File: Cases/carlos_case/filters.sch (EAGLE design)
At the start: 93 parts, among them IC1 NE5532N, IC2 NE5532N, IC3 NE5532N, IC4 NE5532N, IC5 NE5532N, IC6 NE5532N, IC7 NE5532N, J1 3_PIN_AMPCONN, J2 4_PIN_AMPCONN

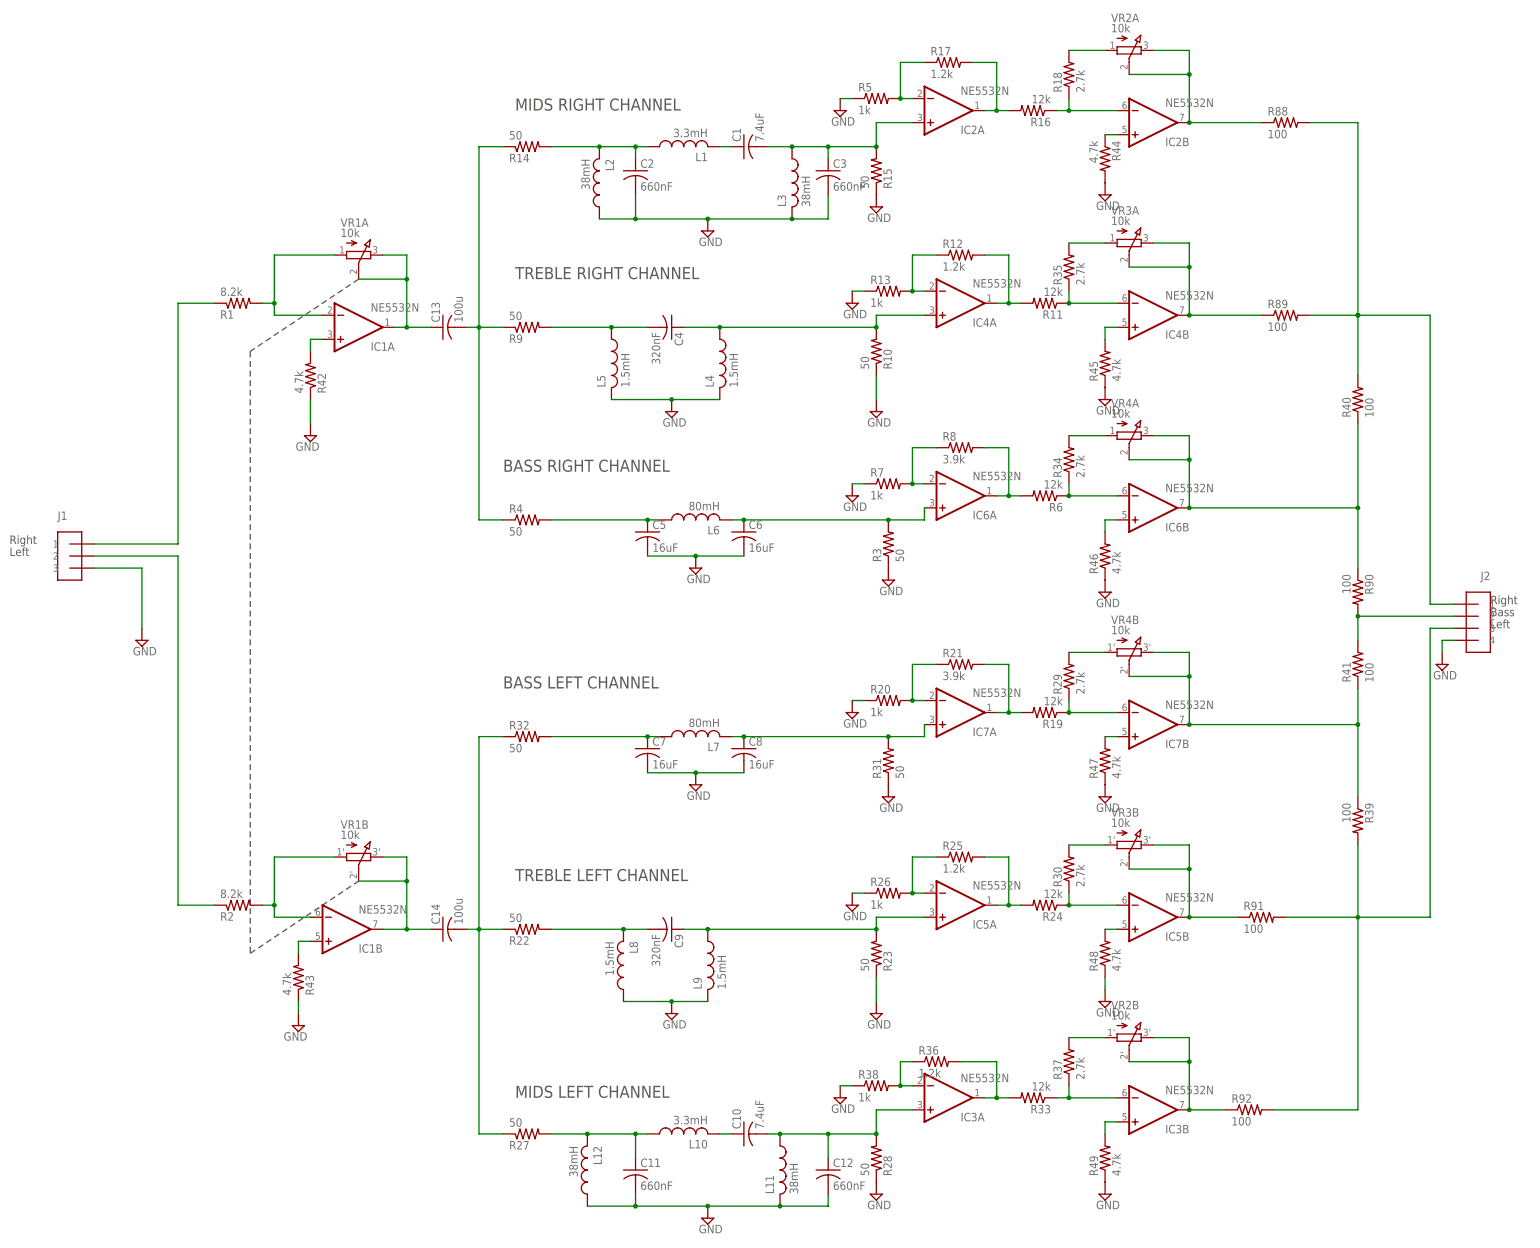
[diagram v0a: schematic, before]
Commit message: added folder for my case
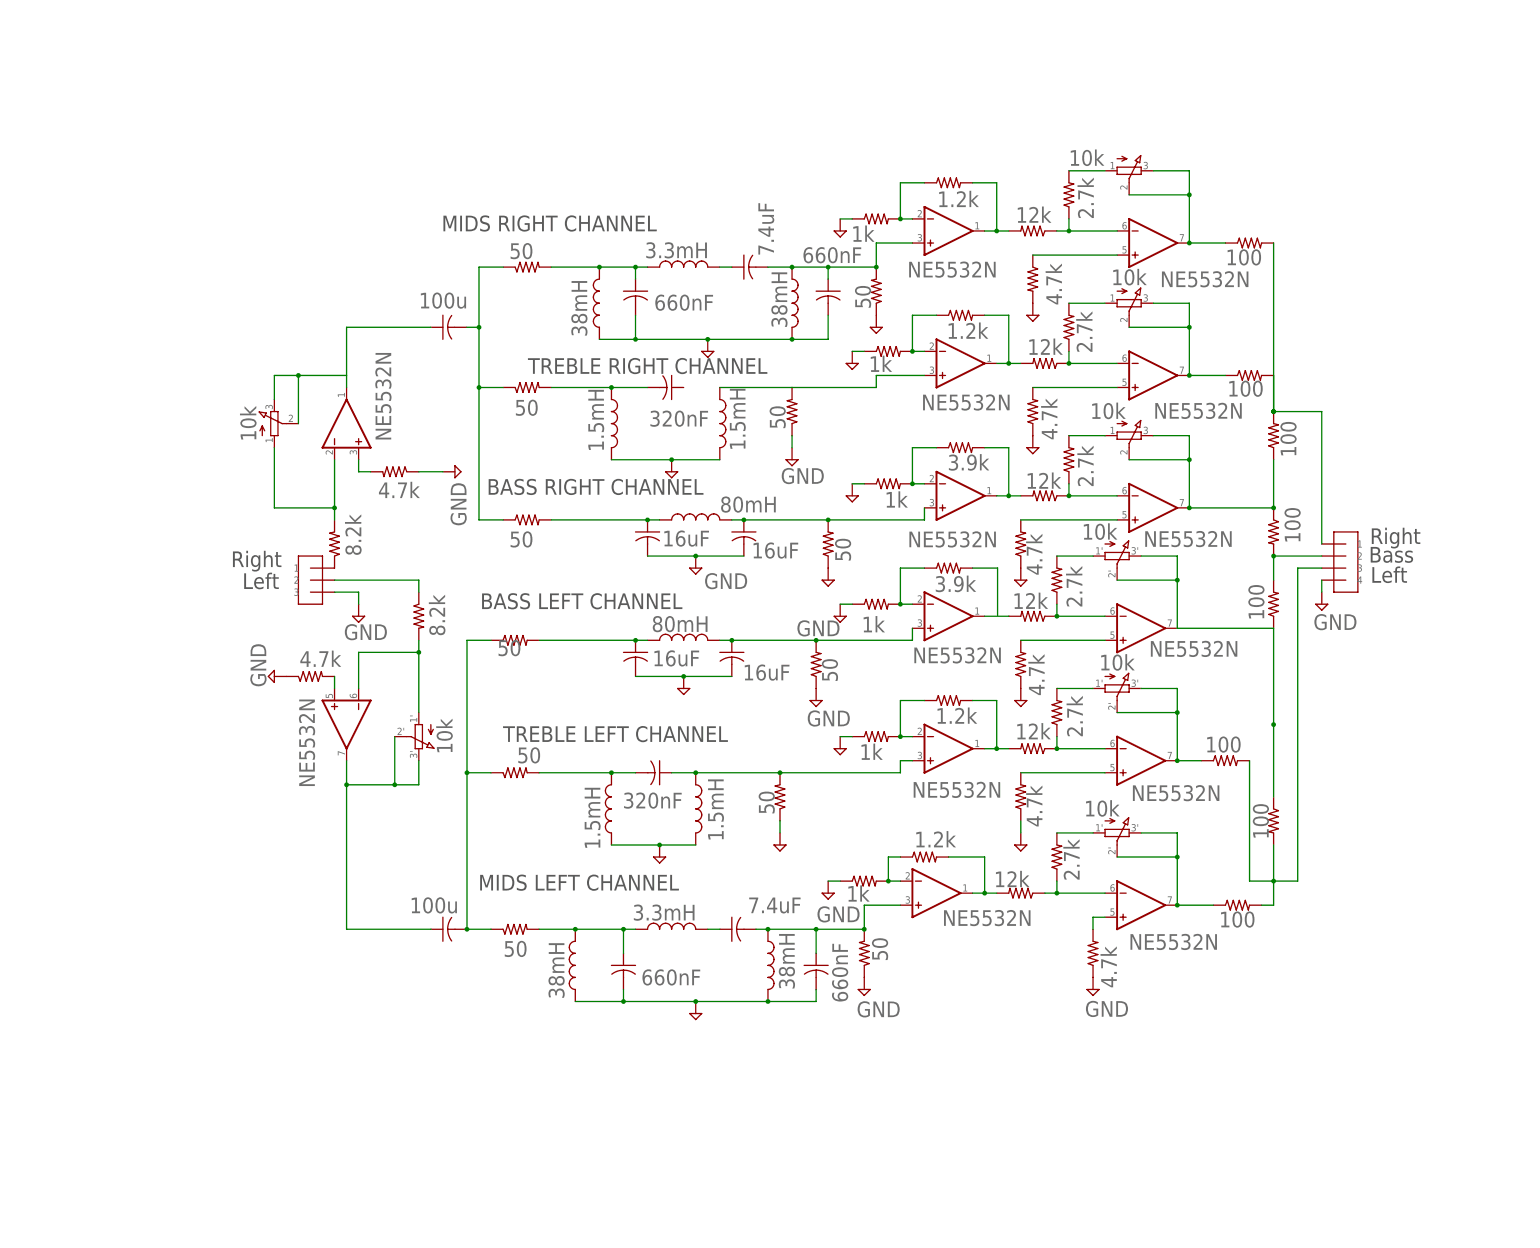
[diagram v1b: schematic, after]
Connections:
- new net N$10: IC7A.OUT, R19.2
- net N$43: no longer IC7A.OUT, R19.2
- net N$63: no longer C4.1
